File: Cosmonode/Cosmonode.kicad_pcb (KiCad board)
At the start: 2 copper layers, 52.7 x 34.3 mm, 51 parts, among them J1 CONN_01X12, J10 WEEE_Logo, J11 Aloes_Logo, J12 Aloes_mini_Logo, J13 CONN_01X05, J14 GS2, J2 CONN_01X12, J3 GS2, J4 OSHW, J5 CONN_01X02, J6 GS2, J8 USB_OTG, J9 GS2, P1 COAX, SW1 SW_DIP_x01, U1 ATMEGA328P-AU, U2 RFM69CW, U3 RN2483, U5 XC6206P332MR, U6 ATSHA204, U7 MCP73811T-420I/OT, Y1 Crystal_GND2

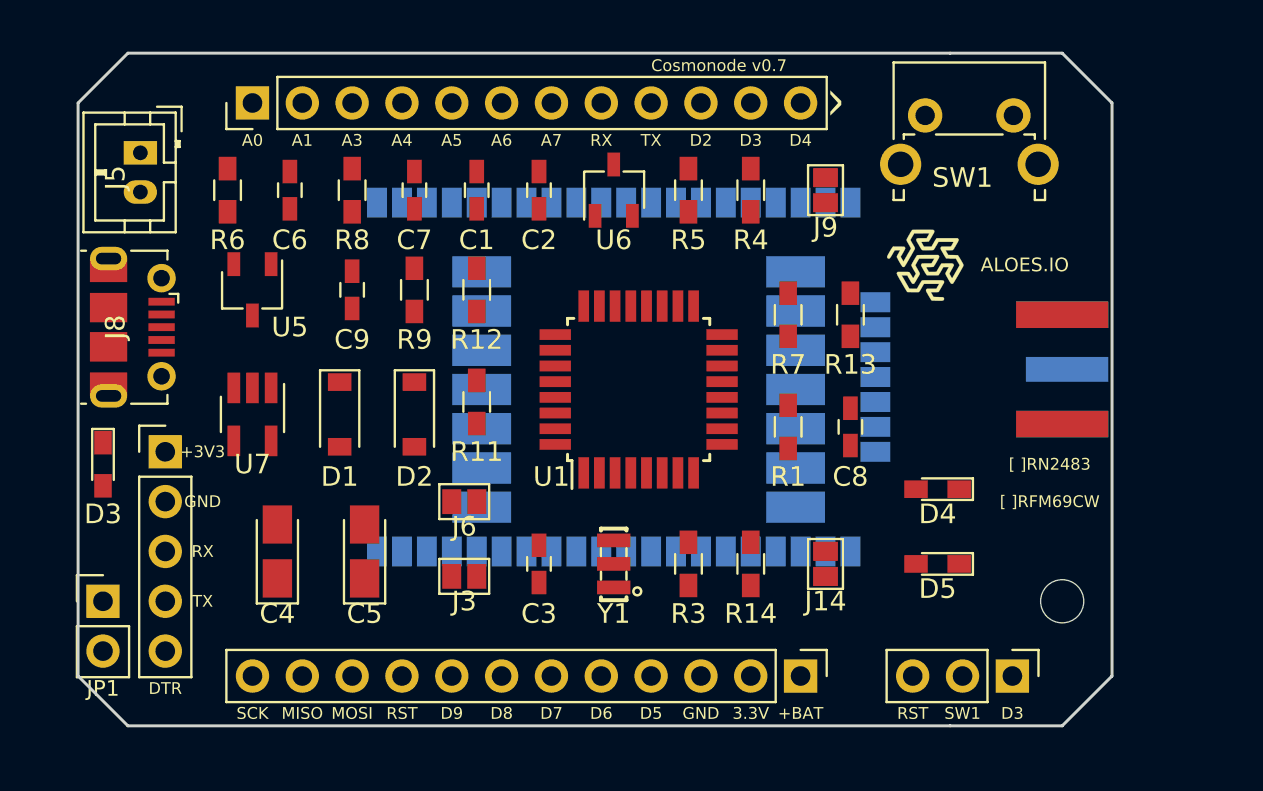
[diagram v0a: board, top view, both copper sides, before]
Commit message: fix and update
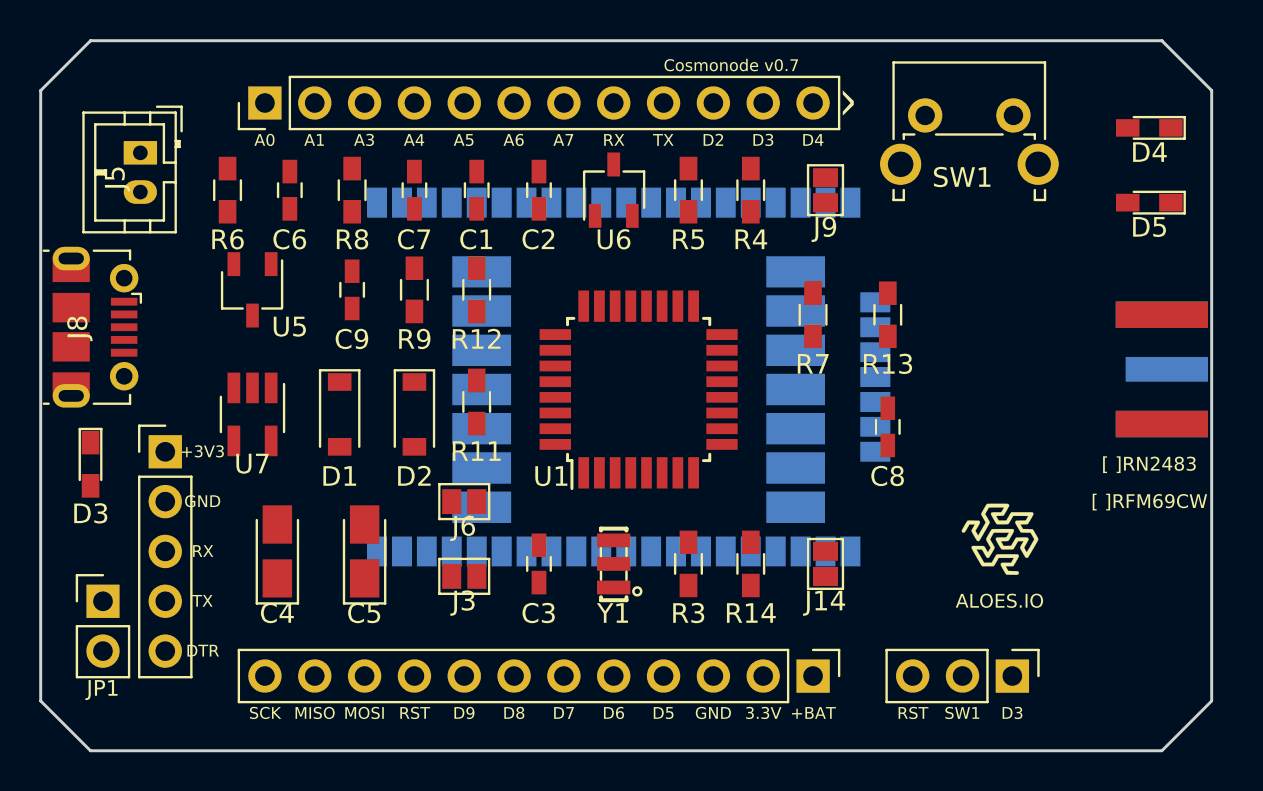
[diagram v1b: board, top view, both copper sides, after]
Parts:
- removed MK1: Mounting_Hole, Mounting_Holes:MountingHole_2.2mm_M2_ISO14580
- removed R1: 10k, Resistors_SMD:R_0603_HandSoldering
- moved D4 21.3 mm to (200.7, 81.3)
- moved D5 21.3 mm to (200.7, 85.1)
- moved J12 14.5 mm to (193.0, 102.2)
- moved P1 5.08 mm to (201.3, 90.8)
- moved C8 1.91 mm to (187.3, 96.5)
- moved J11 1.91 mm to (155.6, 86.4)
- moved J4 1.91 mm to (155.6, 95.2)
- moved J8 1.91 mm to (146.1, 91.4)
- moved R13 1.91 mm to (187.3, 90.8)
- moved J10 1.27 mm to (155.6, 102.2)
- moved R7 1.27 mm to (183.5, 90.8)
- moved D3 0.63 mm to (146.7, 98.4)
- moved J1 0.63 mm to (155.6, 80.0)
- moved J2 0.63 mm to (183.5, 109.2)
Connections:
- net /RADIO_RESET renamed /RN2483_RST
- J3 pad 2: D9 -> D10
- J6 pad 2: D11/MOSI -> D8
- U3 pad 6: D11/MOSI -> D8
- U3 pad 7: D10 -> D9
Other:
- board size 52.7 x 34.3 mm -> 59.7 x 36.2 mm
